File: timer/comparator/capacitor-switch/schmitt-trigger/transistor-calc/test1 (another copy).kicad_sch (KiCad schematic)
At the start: 10 parts, among them Q1 NPN, Q2 NPN

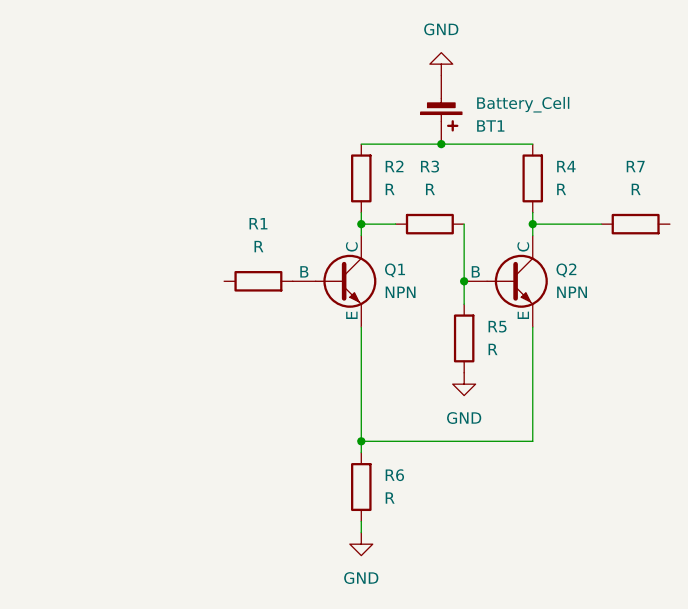
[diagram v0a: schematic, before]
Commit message: add/fix
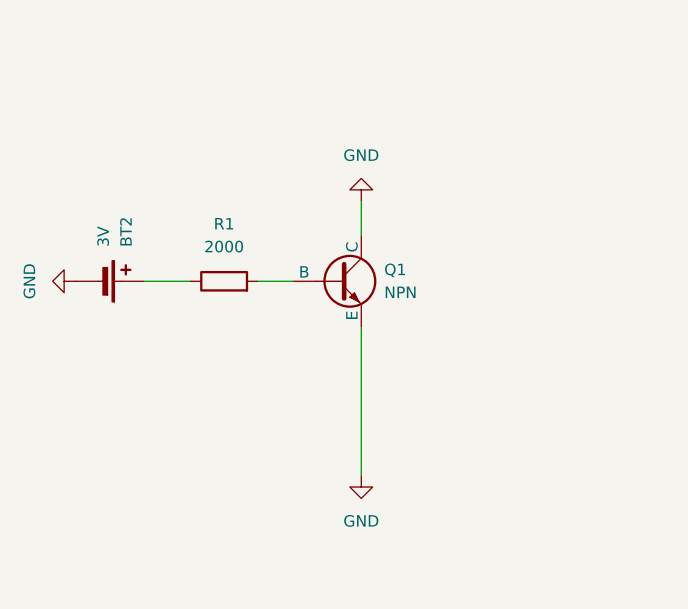
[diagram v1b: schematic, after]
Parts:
- removed BT1: Battery_Cell, symbol Device:Battery_Cell
- removed Q2: NPN, symbol Simulation_SPICE:NPN
- removed R2, R3, R4, R5, R6, R7: R, symbol Device:R
- added BT2: 3V, symbol Device:Battery_Cell
- R1: value R -> 2000
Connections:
- net GND: now also Q1.1 (C), Q1.3 (E), BT2.2 (-)
- net at R1.1: now also BT2.1 (+)
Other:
- moved on the sheet: R1
